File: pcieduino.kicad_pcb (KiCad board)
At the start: 2 copper layers, 51 x 30 mm, 32 parts, among them IC1 ATMEGA328P-A, J1 PCIE-MINI, J3 POWER, J4 ISP, J5 ANALOG, P1 DIGITAL, SW1 SW_PUSH, U1 MCP2200, X1 12MHz, X2 8MHz

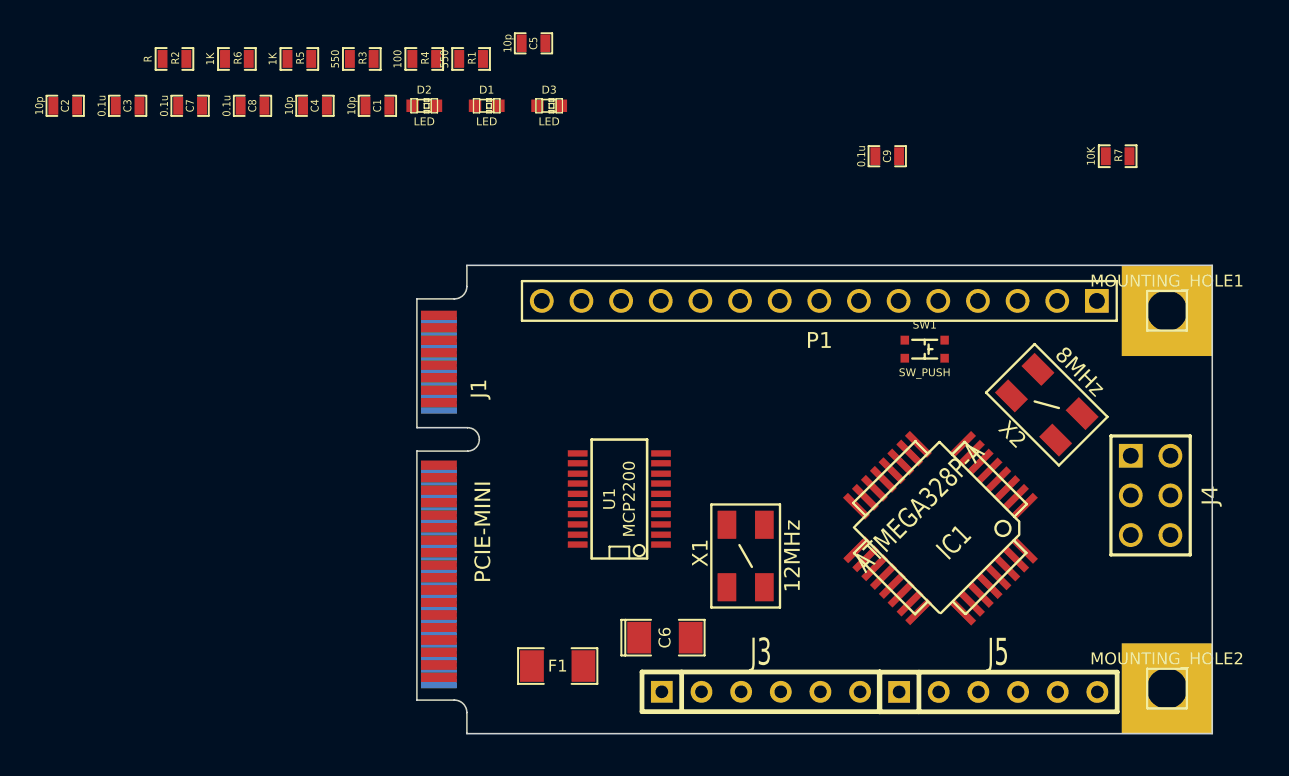
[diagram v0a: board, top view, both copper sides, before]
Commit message: more progress on 01/03
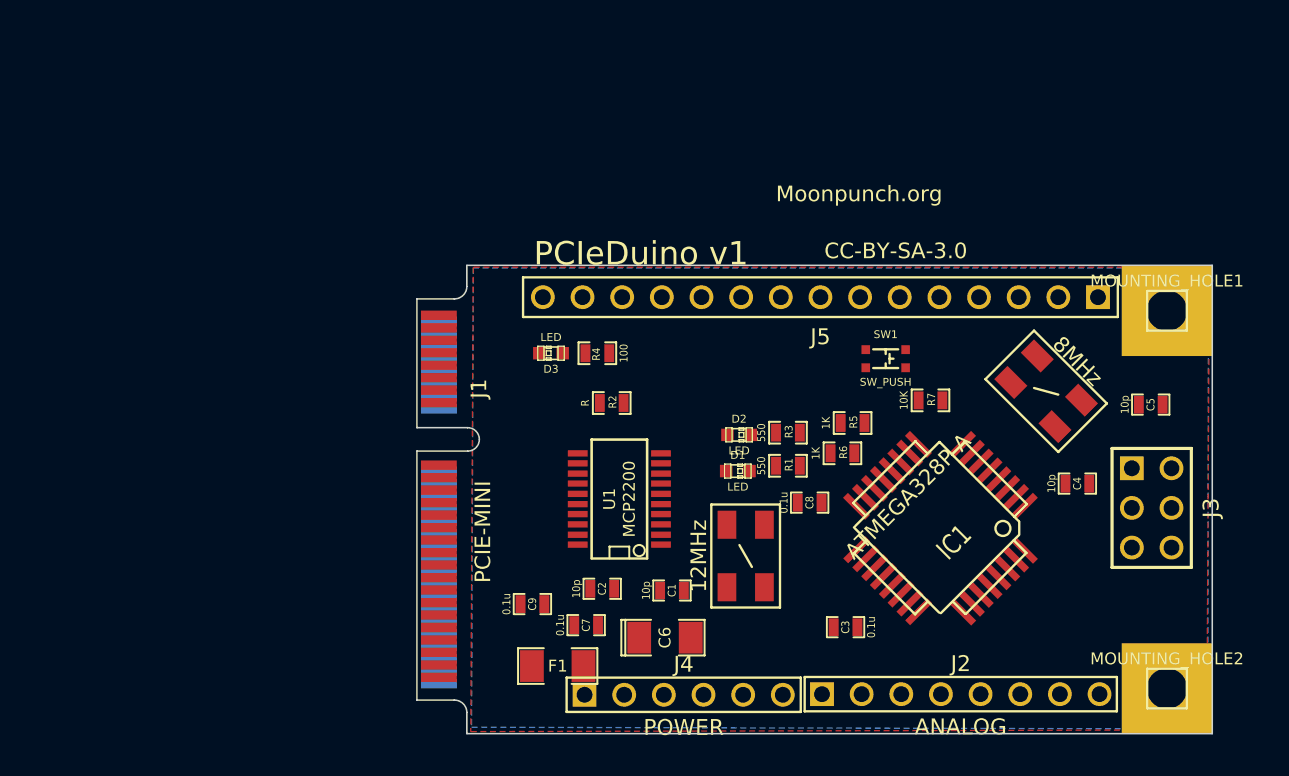
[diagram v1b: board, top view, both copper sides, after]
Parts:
- removed P1: DIGITAL, PIN_ARRAY_15x1
- added J2: ANALOG, pin_array_8x1, F.Cu at (168.8, 113.3)
- J3: value POWER -> ISP; footprint SIL-6 -> pin_array_3x2
- J4: value ISP -> POWER; footprint pin_array_3x2 -> pin_array_6x1
- J5: value ANALOG -> DIGITAL; footprint SIL-6 -> PIN_ARRAY_15x1
- moved C3 56.8 mm to (161.4, 109.0), turned to 180 degrees
- moved C4 54.5 mm to (176.3, 99.8)
- moved R6 46.3 mm to (161.2, 97.9)
- moved C2 46.3 mm to (145.8, 106.6)
- moved C5 45.8 mm to (181.0, 94.8)
- moved C8 43.8 mm to (159.1, 101.0)
- moved R5 42.4 mm to (161.9, 95.9)
- moved C7 41.8 mm to (144.8, 108.9)
- moved C9 36.6 mm to (141.4, 107.5)
- moved C1 36.3 mm to (150.3, 106.7)
- moved R3 36.3 mm to (157.8, 96.6)
- moved R2 35.6 mm to (146.5, 94.7)
- moved R1 33.0 mm to (157.8, 98.7)
- moved J4 32.5 mm to (151.1, 113.3), turned to 0 degrees
- moved D2 29.2 mm to (154.6, 96.7)
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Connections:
- IC1 pad 19: (no net) -> /A6
- IC1 pad 22: (no net) -> /A7
- J3 pad 1: /RESET -> /D12/MISO
- J3 pad 3: VCC -> /D13/SCK
- J3 pad 4: GND -> /D11/MOSI
- J3 pad 5: GND -> /RESET
- J3 pad 6: /AREF -> GND
- J4 pad 1: /D12/MISO -> /RESET
- J4 pad 3: /D13/SCK -> VCC
- J4 pad 4: /D11/MOSI -> GND
- J4 pad 5: /RESET -> GND
- J4 pad 6: GND -> /AREF
- J5 pad 1: /A0 -> N-0000035
- J5 pad 2: /A1 -> N-0000034
- J5 pad 3: /A2 -> /D2
- J5 pad 4: /A3 -> /D3
- J5 pad 5: /A4 -> /D4
- J5 pad 6: /A5 -> /D5
- R5 pad 2: N-0000047 (its old number) -> N-0000035
- R6 pad 2: N-0000048 -> N-0000034
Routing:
- added copper zone on F.Cu, net GND
- added copper zone on B.Cu, net VCC
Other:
- board text added: "CC-BY-SA-3.0"
- board text added: "Moonpunch.org"
- board text added: "PCIeDuino v1"
